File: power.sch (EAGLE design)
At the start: 52 parts, among them IC2 7805TV

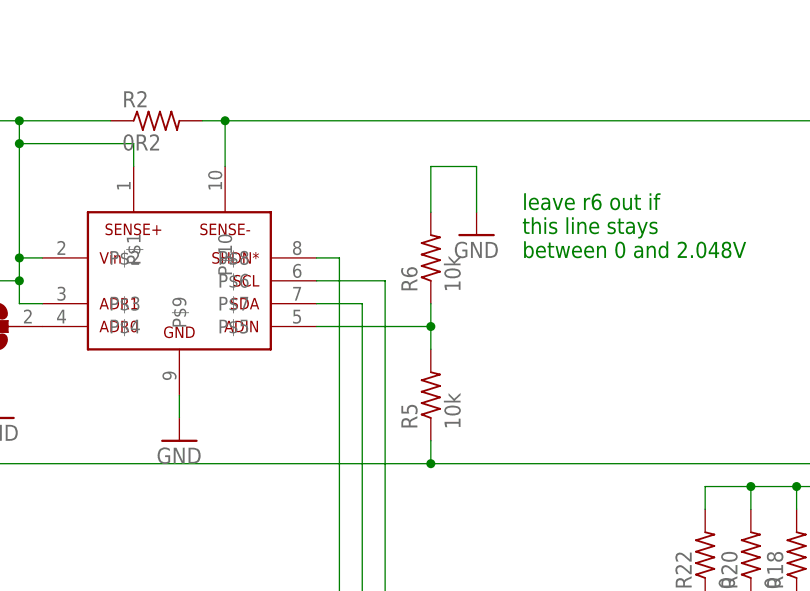
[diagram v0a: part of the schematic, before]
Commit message: still working on it
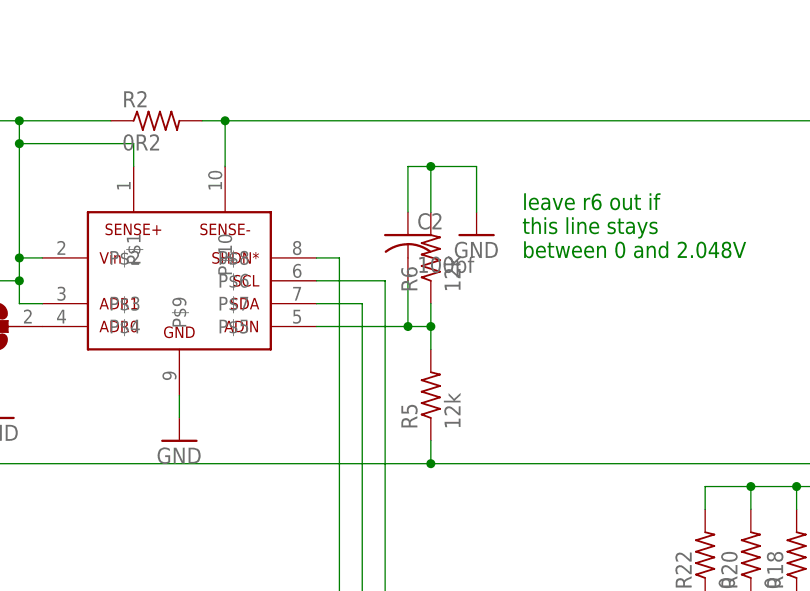
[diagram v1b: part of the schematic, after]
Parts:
- added C2: 100pf, rcl:C-USC0603K
- R5, R6: value 10k -> 12k
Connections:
- net GND: now also C2.1
- net N$30: now also C2.2
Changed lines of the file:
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@@
 <part name="SJ5" library="jumper" deviceset="SJ2W" device=""/>
 <part name="SJ6" library="jumper" deviceset="SJ2W" device=""/>
-<part name="R5" library="rcl" deviceset="R-US_" device="R0603" value="10k"/>
-<part name="R6" library="rcl" deviceset="R-US_" device="R0603" value="10k"/>
+<part name="R5" library="rcl" deviceset="R-US_" device="R0603" value="12k"/>
+<part name="R6" library="rcl" deviceset="R-US_" device="R0603" value="12k"/>
 <part name="GND5" library="supply1" deviceset="GND" device=""/>
 <part name="R7" library="rcl" deviceset="R-US_" device="R0603" value="0"/>
@@
 <part name="R29" library="rcl" deviceset="R-US_" device="R0603" value="0"/>
 <part name="R30" library="rcl" deviceset="R-US_" device="R0603" value="0"/>
+<part name="C2" library="rcl" deviceset="C-US" device="C0603K" value="100pf"/>
 </parts>
 <sheets>
@@
 <instance part="R29" gate="G$1" x="33.02" y="33.02" rot="R90"/>
 <instance part="R30" gate="G$1" x="30.48" y="48.26" rot="R90"/>
+<instance part="C2" gate="G$1" x="-25.4" y="83.82"/>
 </instances>
 <busses>
@@
 <wire x1="-22.86" y1="91.44" x2="-17.78" y2="91.44" width="0.1524" layer="91"/>
 <wire x1="-17.78" y1="91.44" x2="-17.78" y2="86.36" width="0.1524" layer="91"/>
+<pinref part="C2" gate="G$1" pin="1"/>
+<wire x1="-25.4" y1="86.36" x2="-25.4" y2="91.44" width="0.1524" layer="91"/>
+<wire x1="-25.4" y1="91.44" x2="-22.86" y2="91.44" width="0.1524" layer="91"/>
+<junction x="-22.86" y="91.44"/>
 </segment>
 <segment>
@@
 <pinref part="U$1" gate="G$1" pin="P$5"/>
 <pinref part="R6" gate="G$1" pin="1"/>
-<wire x1="-35.56" y1="73.66" x2="-22.86" y2="73.66" width="0.1524" layer="91"/>
+<wire x1="-35.56" y1="73.66" x2="-25.4" y2="73.66" width="0.1524" layer="91"/>
+<wire x1="-25.4" y1="73.66" x2="-22.86" y2="73.66" width="0.1524" layer="91"/>
 <wire x1="-22.86" y1="73.66" x2="-22.86" y2="76.2" width="0.1524" layer="91"/>
 <pinref part="R5" gate="G$1" pin="2"/>
 <wire x1="-22.86" y1="73.66" x2="-22.86" y2="71.12" width="0.1524" layer="91"/>
 <junction x="-22.86" y="73.66"/>
-</segment>
-</net>
+<pinref part="C2" gate="G$1" pin="2"/>
+<wire x1="-25.4" y1="78.74" x2="-25.4" y2="73.66" width="0.1524" layer="91"/>
+<junction x="-25.4" y="73.66"/>
+</segment>
+</net>

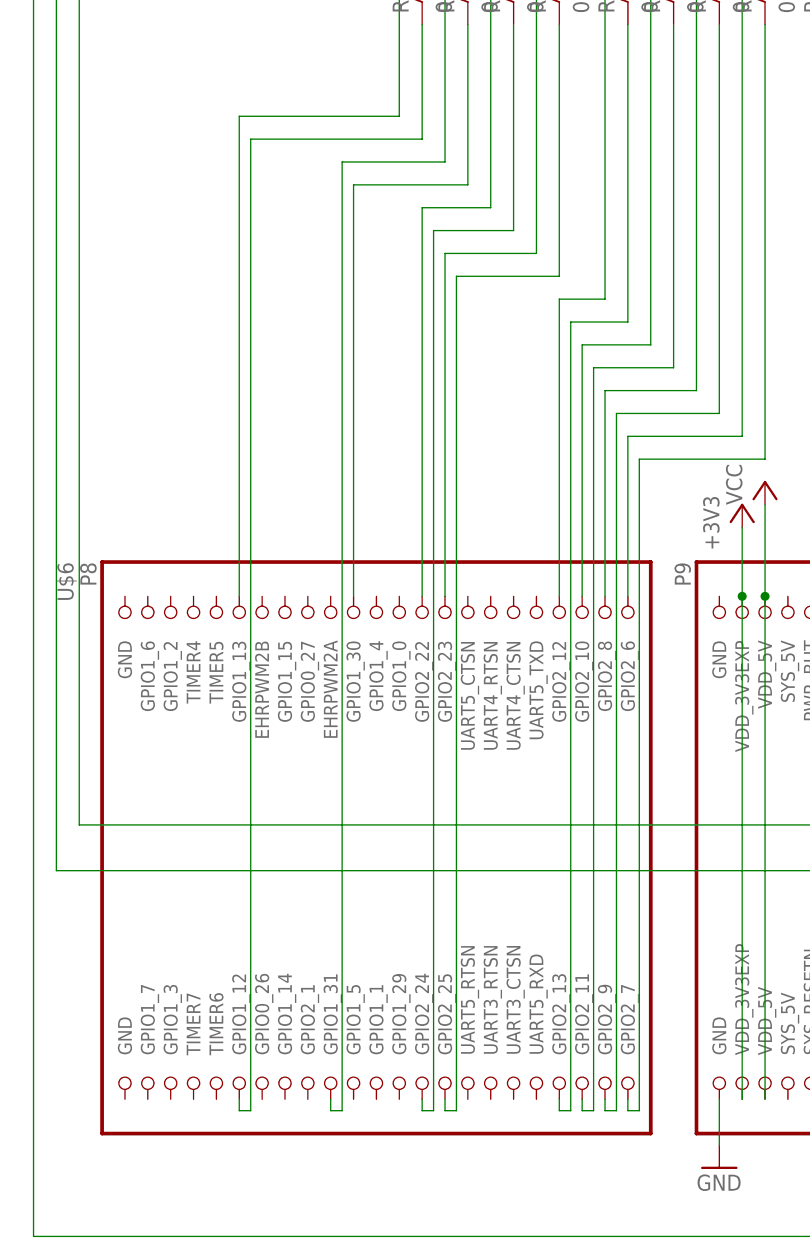
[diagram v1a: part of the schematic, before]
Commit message: almost there
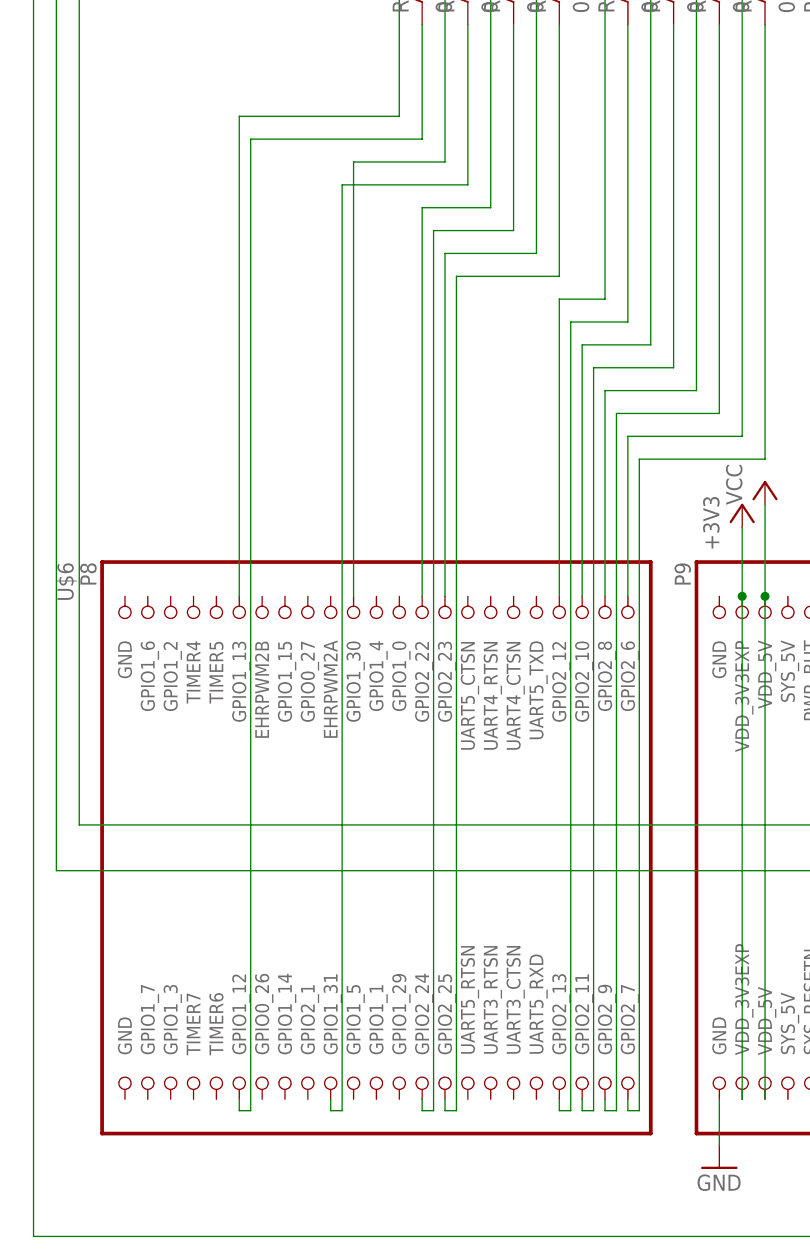
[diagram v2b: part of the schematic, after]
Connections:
- removed net N$39: R19.1, U$6.GPIO1_30
- new net N$36: R19.1, U$6.GPIO1_31
- net N$38: now also U$6.GPIO1_30; no longer U$6.GPIO1_31
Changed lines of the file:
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@@
-</segment>
-</net>
-<net name="N$38" class="0">
-<segment>
-<pinref part="U$6" gate="G$1" pin="GPIO1_31"/>
-<wire x1="0" y1="-91.44" x2="0" y2="-92.71" width="0.1524" layer="91"/>
-<wire x1="0" y1="-92.71" x2="1.27" y2="-92.71" width="0.1524" layer="91"/>
-<wire x1="1.27" y1="-92.71" x2="1.27" y2="12.7" width="0.1524" layer="91"/>
-<wire x1="1.27" y1="12.7" x2="12.7" y2="12.7" width="0.1524" layer="91"/>
-<pinref part="R20" gate="G$1" pin="1"/>
-<wire x1="12.7" y1="12.7" x2="12.7" y2="43.18" width="0.1524" layer="91"/>
-</segment>
-</net>
-<net name="N$39" class="0">
-<segment>
-<pinref part="U$6" gate="G$1" pin="GPIO1_30"/>
-<wire x1="2.54" y1="-35.56" x2="2.54" y2="10.16" width="0.1524" layer="91"/>
-<wire x1="2.54" y1="10.16" x2="15.24" y2="10.16" width="0.1524" layer="91"/>
-<pinref part="R19" gate="G$1" pin="1"/>
-<wire x1="15.24" y1="10.16" x2="15.24" y2="27.94" width="0.1524" layer="91"/>
 </segment>
 </net>
@@
 </segment>
 </net>
-<net name="N$13" class="0">
+<net name="N$27" class="0">
 <segment>
-<wire x1="-8.89" y1="15.24" x2="10.16" y2="15.24" width="0.1524" layer="91"/>
-<pinref part="R21" gate="G$1" pin="1"/>
-<wire x1="10.16" y1="15.24" x2="10.16" y2="27.94" width="0.1524" layer="91"/>
 <pinref part="U$6" gate="G$1" pin="GPIO1_12"/>
 <wire x1="-10.16" y1="-91.44" x2="-10.16" y2="-92.71" width="0.1524" layer="91"/>
 <wire x1="-10.16" y1="-92.71" x2="-8.89" y2="-92.71" width="0.1524" layer="91"/>
 <wire x1="-8.89" y1="-92.71" x2="-8.89" y2="15.24" width="0.1524" layer="91"/>
+<pinref part="R21" gate="G$1" pin="1"/>
+<wire x1="10.16" y1="15.24" x2="10.16" y2="27.94" width="0.1524" layer="91"/>
+<wire x1="-8.89" y1="15.24" x2="10.16" y2="15.24" width="0.1524" layer="91"/>
 </segment>
 </net>
+<net name="N$36" class="0">
+<segment>
+<pinref part="R19" gate="G$1" pin="1"/>
+<wire x1="15.24" y1="10.16" x2="15.24" y2="27.94" width="0.1524" layer="91"/>
+<pinref part="U$6" gate="G$1" pin="GPIO1_31"/>
+<wire x1="0" y1="-91.44" x2="0" y2="-92.71" width="0.1524" layer="91"/>
+<wire x1="0" y1="-92.71" x2="1.27" y2="-92.71" width="0.1524" layer="91"/>
+<wire x1="1.27" y1="10.16" x2="1.27" y2="-92.71" width="0.1524" layer="91"/>
+<wire x1="15.24" y1="10.16" x2="1.27" y2="10.16" width="0.1524" layer="91"/>
+</segment>
+</net>
+<net name="N$38" class="0">
+<segment>
+<pinref part="R20" gate="G$1" pin="1"/>
+<wire x1="12.7" y1="12.7" x2="12.7" y2="43.18" width="0.1524" layer="91"/>
+<pinref part="U$6" gate="G$1" pin="GPIO1_30"/>
+<wire x1="2.54" y1="-35.56" x2="2.54" y2="12.7" width="0.1524" layer="91"/>
+<wire x1="12.7" y1="12.7" x2="2.54" y2="12.7" width="0.1524" layer="91"/>
+</segment>
+</net>

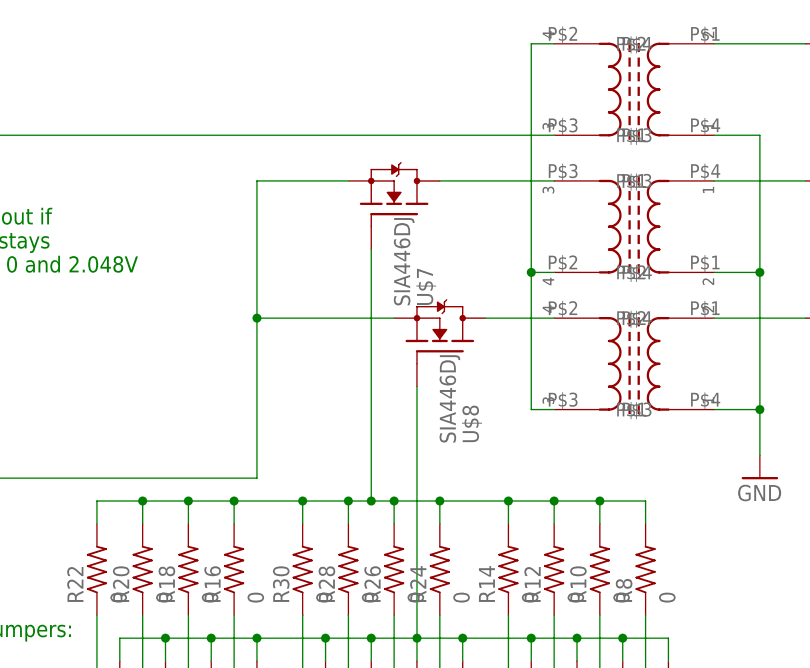
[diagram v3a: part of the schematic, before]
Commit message: LETS HOOK UP THE MOSFETS THE RIGHT WAY, OKAY?
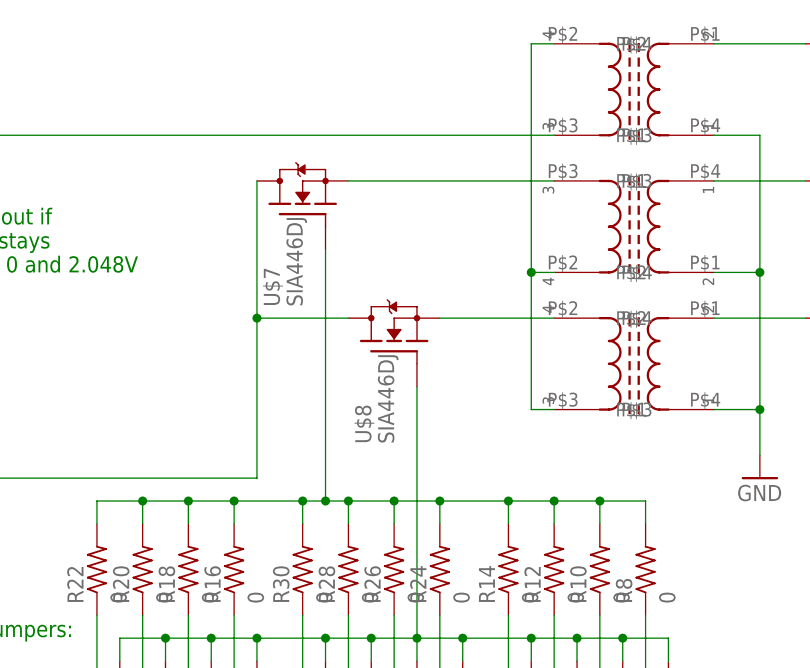
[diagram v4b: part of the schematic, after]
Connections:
- net N$2: now also U$8.S; no longer U$8.D
- net N$3: now also U$7.S; no longer U$7.D
- net N$8: now also U$7.D, U$8.D; no longer U$7.S, U$8.S
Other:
- moved on the sheet: U$7, U$8
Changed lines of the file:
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@@
 <instance part="H1" gate="G$1" x="154.94" y="68.58"/>
 <instance part="GND6" gate="1" x="149.86" y="58.42"/>
-<instance part="U$7" gate="G$1" x="40.64" y="88.9" rot="MR90"/>
-<instance part="U$8" gate="G$1" x="45.72" y="73.66" rot="MR90"/>
+<instance part="U$7" gate="G$1" x="30.48" y="88.9" rot="R90"/>
+<instance part="U$8" gate="G$1" x="40.64" y="73.66" rot="R90"/>
 <instance part="H2" gate="G$1" x="154.94" y="63.5"/>
 <instance part="H3" gate="G$1" x="154.94" y="73.66"/>
@@
 <net name="N$8" class="2">
 <segment>
-<pinref part="U$8" gate="G$1" pin="S"/>
 <wire x1="25.4" y1="58.42" x2="25.4" y2="76.2" width="0.1524" layer="91"/>
-<wire x1="40.64" y1="76.2" x2="25.4" y2="76.2" width="0.1524" layer="91"/>
-<pinref part="U$7" gate="G$1" pin="S"/>
-<wire x1="35.56" y1="91.44" x2="25.4" y2="91.44" width="0.1524" layer="91"/>
-<wire x1="25.4" y1="91.44" x2="25.4" y2="76.2" width="0.1524" layer="91"/>
-<junction x="25.4" y="76.2"/>
 <pinref part="PV-" gate="G$1" pin="MOUNT"/>
+<wire x1="25.4" y1="76.2" x2="25.4" y2="91.44" width="0.1524" layer="91"/>
 <wire x1="-71.12" y1="58.42" x2="-22.86" y2="58.42" width="0.1524" layer="91"/>
 <pinref part="R5" gate="G$1" pin="1"/>
@@
 <wire x1="-22.86" y1="60.96" x2="-22.86" y2="58.42" width="0.1524" layer="91"/>
 <junction x="-22.86" y="58.42"/>
+<pinref part="U$7" gate="G$1" pin="D"/>
+<pinref part="U$8" gate="G$1" pin="D"/>
+<wire x1="25.4" y1="76.2" x2="35.56" y2="76.2" width="0.1524" layer="91"/>
+<junction x="25.4" y="76.2"/>
 </segment>
 </net>
@@
 <wire x1="48.26" y1="-35.56" x2="48.26" y2="-91.44" width="0.1524" layer="91"/>
 <junction x="48.26" y="-35.56"/>
-</segment>
-</net>
-<net name="N$2" class="2">
-<segment>
-<pinref part="U$4" gate="G$1" pin="P$4"/>
-<pinref part="U$8" gate="G$1" pin="D"/>
-<wire x1="58.42" y1="76.2" x2="50.8" y2="76.2" width="0.1524" layer="91"/>
-</segment>
-</net>
-<net name="N$3" class="2">
-<segment>
-<pinref part="U$7" gate="G$1" pin="D"/>
-<pinref part="U$5" gate="G$1" pin="P$3"/>
-<wire x1="45.72" y1="91.44" x2="58.42" y2="91.44" width="0.1524" layer="91"/>
 </segment>
 </net>
@@
 <pinref part="R22" gate="G$1" pin="2"/>
 <wire x1="7.62" y1="53.34" x2="7.62" y2="55.88" width="0.1524" layer="91"/>
-<wire x1="30.48" y1="55.88" x2="35.56" y2="55.88" width="0.1524" layer="91"/>
-<wire x1="35.56" y1="55.88" x2="38.1" y2="55.88" width="0.1524" layer="91"/>
-<wire x1="38.1" y1="55.88" x2="40.64" y2="55.88" width="0.1524" layer="91"/>
+<wire x1="30.48" y1="55.88" x2="33.02" y2="55.88" width="0.1524" layer="91"/>
+<wire x1="33.02" y1="55.88" x2="35.56" y2="55.88" width="0.1524" layer="91"/>
+<wire x1="35.56" y1="55.88" x2="40.64" y2="55.88" width="0.1524" layer="91"/>
 <wire x1="40.64" y1="55.88" x2="45.72" y2="55.88" width="0.1524" layer="91"/>
 <pinref part="R24" gate="G$1" pin="2"/>
@@
 <junction x="53.34" y="55.88"/>
 <pinref part="U$7" gate="G$1" pin="G"/>
-<wire x1="38.1" y1="83.82" x2="38.1" y2="55.88" width="0.1524" layer="91"/>
-<junction x="38.1" y="55.88"/>
+<wire x1="33.02" y1="55.88" x2="33.02" y2="83.82" width="0.1524" layer="91"/>
+<junction x="33.02" y="55.88"/>
 </segment>
 </net>
@@
 </segment>
 </net>
+<net name="N$2" class="0">
+<segment>
+<pinref part="U$8" gate="G$1" pin="S"/>
+<pinref part="U$4" gate="G$1" pin="P$4"/>
+<wire x1="45.72" y1="76.2" x2="58.42" y2="76.2" width="0.1524" layer="91"/>
+</segment>
+</net>
+<net name="N$3" class="0">
+<segment>
+<pinref part="U$7" gate="G$1" pin="S"/>
+<pinref part="U$5" gate="G$1" pin="P$3"/>
+<wire x1="35.56" y1="91.44" x2="58.42" y2="91.44" width="0.1524" layer="91"/>
+</segment>
+</net>

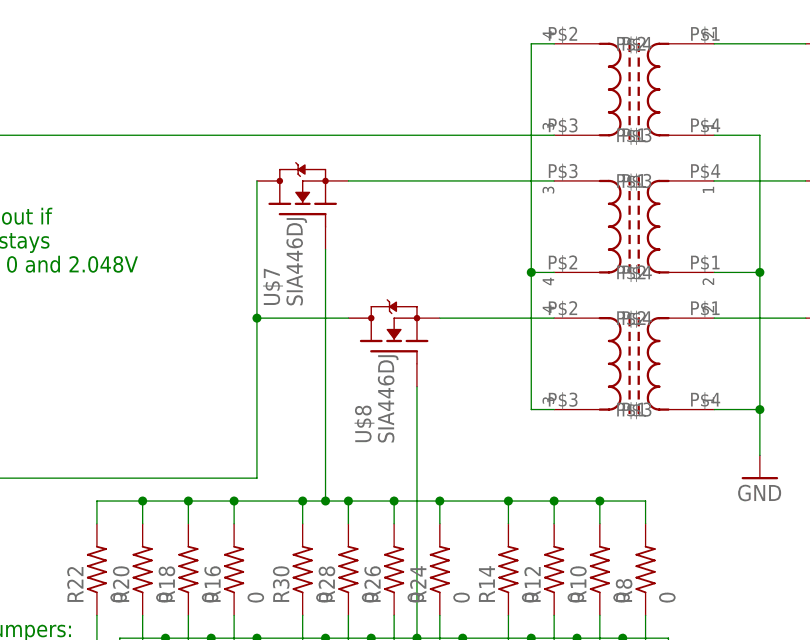
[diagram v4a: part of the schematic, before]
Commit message: i'm pretty sure i had the FETs in the right way in the first place, actually...
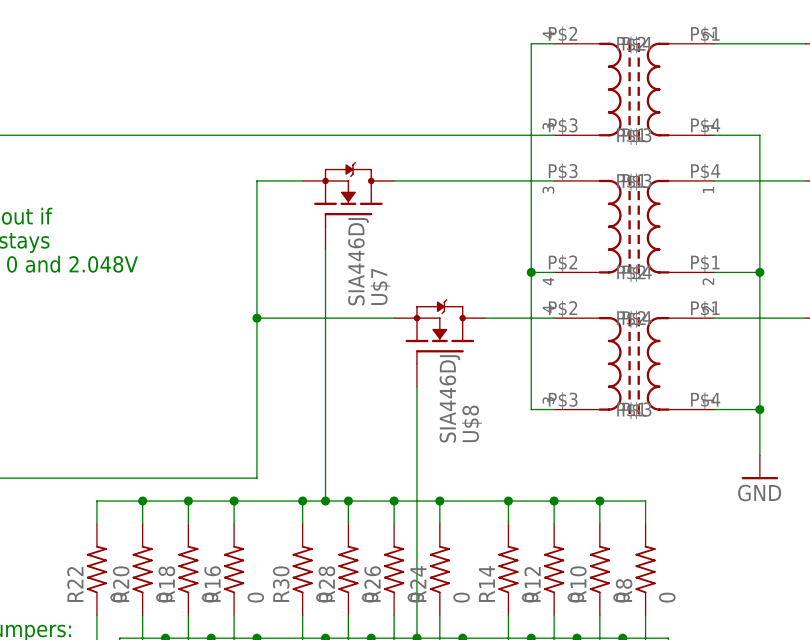
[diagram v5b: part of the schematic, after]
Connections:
- net N$2: now also U$5.P$3, U$7.D; no longer U$4.P$4, U$8.S
- net N$3: now also U$4.P$4, U$8.D; no longer U$5.P$3, U$7.S
- net N$8: now also U$7.S, U$8.S; no longer U$7.D, U$8.D
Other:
- moved on the sheet: U$7, U$8
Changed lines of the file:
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@@
 <instance part="H1" gate="G$1" x="154.94" y="68.58"/>
 <instance part="GND6" gate="1" x="149.86" y="58.42"/>
-<instance part="U$7" gate="G$1" x="30.48" y="88.9" rot="R90"/>
-<instance part="U$8" gate="G$1" x="40.64" y="73.66" rot="R90"/>
+<instance part="U$7" gate="G$1" x="35.56" y="88.9" rot="MR90"/>
+<instance part="U$8" gate="G$1" x="45.72" y="73.66" rot="MR90"/>
 <instance part="H2" gate="G$1" x="154.94" y="63.5"/>
 <instance part="H3" gate="G$1" x="154.94" y="73.66"/>
@@
 <net name="N$8" class="2">
 <segment>
-<wire x1="25.4" y1="58.42" x2="25.4" y2="76.2" width="0.1524" layer="91"/>
 <pinref part="PV-" gate="G$1" pin="MOUNT"/>
-<wire x1="25.4" y1="76.2" x2="25.4" y2="91.44" width="0.1524" layer="91"/>
 <wire x1="-71.12" y1="58.42" x2="-22.86" y2="58.42" width="0.1524" layer="91"/>
 <pinref part="R5" gate="G$1" pin="1"/>
@@
 <wire x1="-22.86" y1="60.96" x2="-22.86" y2="58.42" width="0.1524" layer="91"/>
 <junction x="-22.86" y="58.42"/>
-<pinref part="U$7" gate="G$1" pin="D"/>
-<pinref part="U$8" gate="G$1" pin="D"/>
-<wire x1="25.4" y1="76.2" x2="35.56" y2="76.2" width="0.1524" layer="91"/>
+<pinref part="U$8" gate="G$1" pin="S"/>
+<wire x1="40.64" y1="76.2" x2="25.4" y2="76.2" width="0.1524" layer="91"/>
+<wire x1="25.4" y1="76.2" x2="25.4" y2="58.42" width="0.1524" layer="91"/>
+<pinref part="U$7" gate="G$1" pin="S"/>
+<wire x1="30.48" y1="91.44" x2="25.4" y2="91.44" width="0.1524" layer="91"/>
+<wire x1="25.4" y1="91.44" x2="25.4" y2="76.2" width="0.1524" layer="91"/>
 <junction x="25.4" y="76.2"/>
 </segment>
@@
 <net name="N$2" class="0">
 <segment>
-<pinref part="U$8" gate="G$1" pin="S"/>
+<pinref part="U$7" gate="G$1" pin="D"/>
+<pinref part="U$5" gate="G$1" pin="P$3"/>
+<wire x1="40.64" y1="91.44" x2="58.42" y2="91.44" width="0.1524" layer="91"/>
+</segment>
+</net>
+<net name="N$3" class="0">
+<segment>
+<pinref part="U$8" gate="G$1" pin="D"/>
 <pinref part="U$4" gate="G$1" pin="P$4"/>
-<wire x1="45.72" y1="76.2" x2="58.42" y2="76.2" width="0.1524" layer="91"/>
-</segment>
-</net>
-<net name="N$3" class="0">
-<segment>
-<pinref part="U$7" gate="G$1" pin="S"/>
-<pinref part="U$5" gate="G$1" pin="P$3"/>
-<wire x1="35.56" y1="91.44" x2="58.42" y2="91.44" width="0.1524" layer="91"/>
-</segment>
-</net>
+<wire x1="50.8" y1="76.2" x2="58.42" y2="76.2" width="0.1524" layer="91"/>
+</segment>
+</net>
